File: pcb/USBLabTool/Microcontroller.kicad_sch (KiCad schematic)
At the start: 25 parts, among them J1 Conn_01x06_Pin, J2 Conn_02x12_Odd_Even, SW1 TS02-66-73-BK-100-SCR-D, U12 STM32H562VGTx, Y1 32.768kHz, Y2 NX2016SA-25M-EXS00A-CS08742

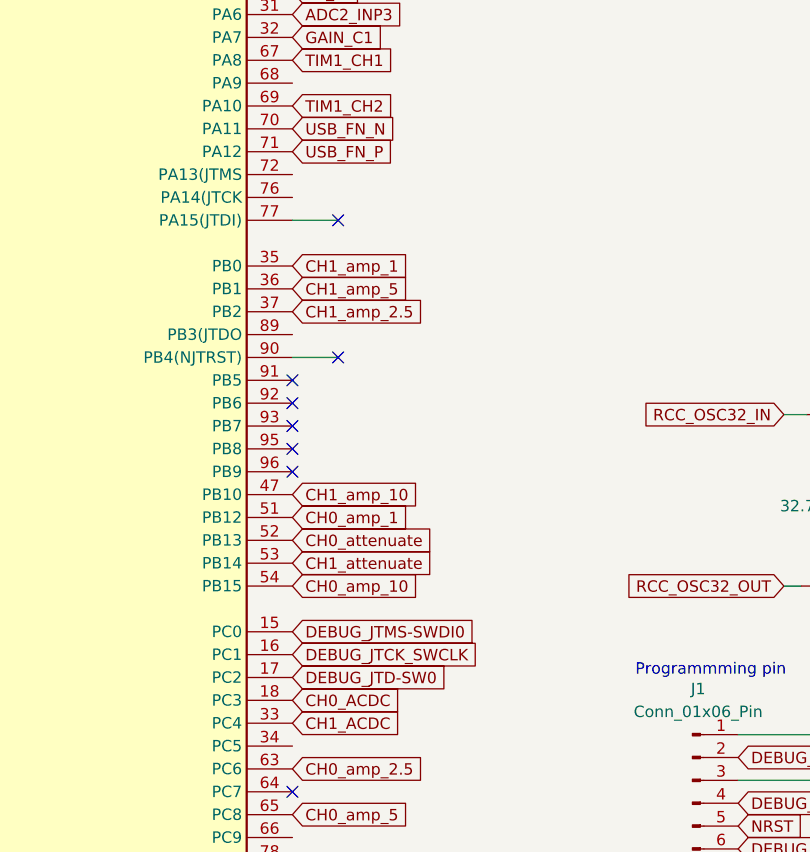
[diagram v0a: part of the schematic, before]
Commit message: reposition a few things
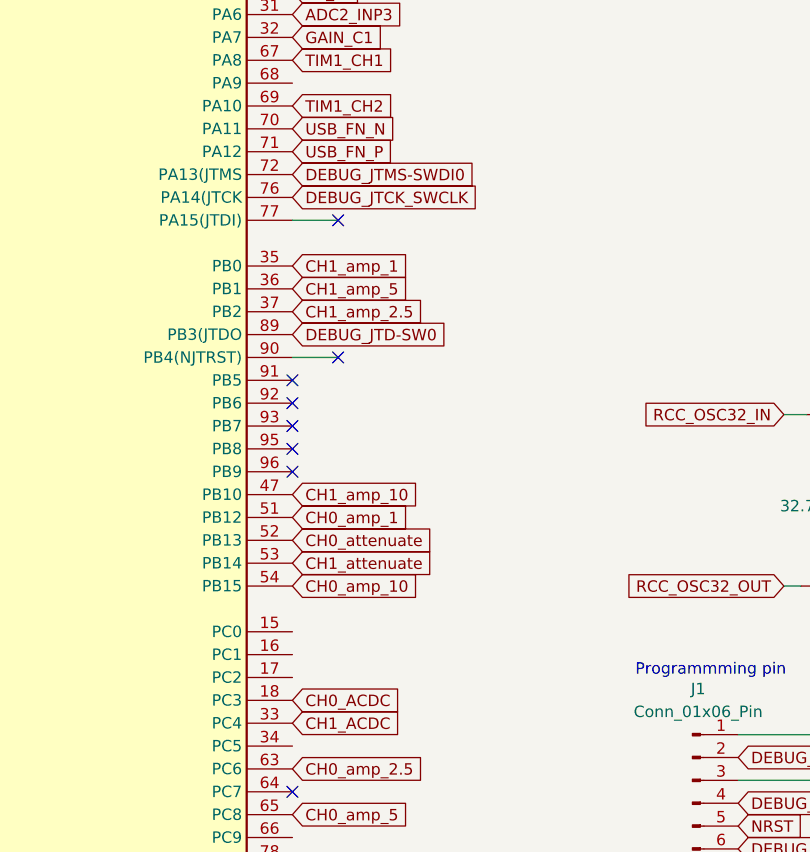
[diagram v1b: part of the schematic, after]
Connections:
- net DEBUG_JTCK_SWCLK: now also U12.76 (PA14(JTCK); no longer U12.16 (PC1)
- net DEBUG_JTD-SW0: now also U12.89 (PB3(JTDO); no longer U12.17 (PC2)
- net DEBUG_JTMS-SWDI0: now also U12.72 (PA13(JTMS); no longer U12.15 (PC0)
